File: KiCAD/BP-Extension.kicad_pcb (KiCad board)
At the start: 2 copper layers, 19.8 x 49.3 mm, 7 parts, among them P1 CONN_01X06, SW1 SW_Push, U1 BP, U2 RFM69

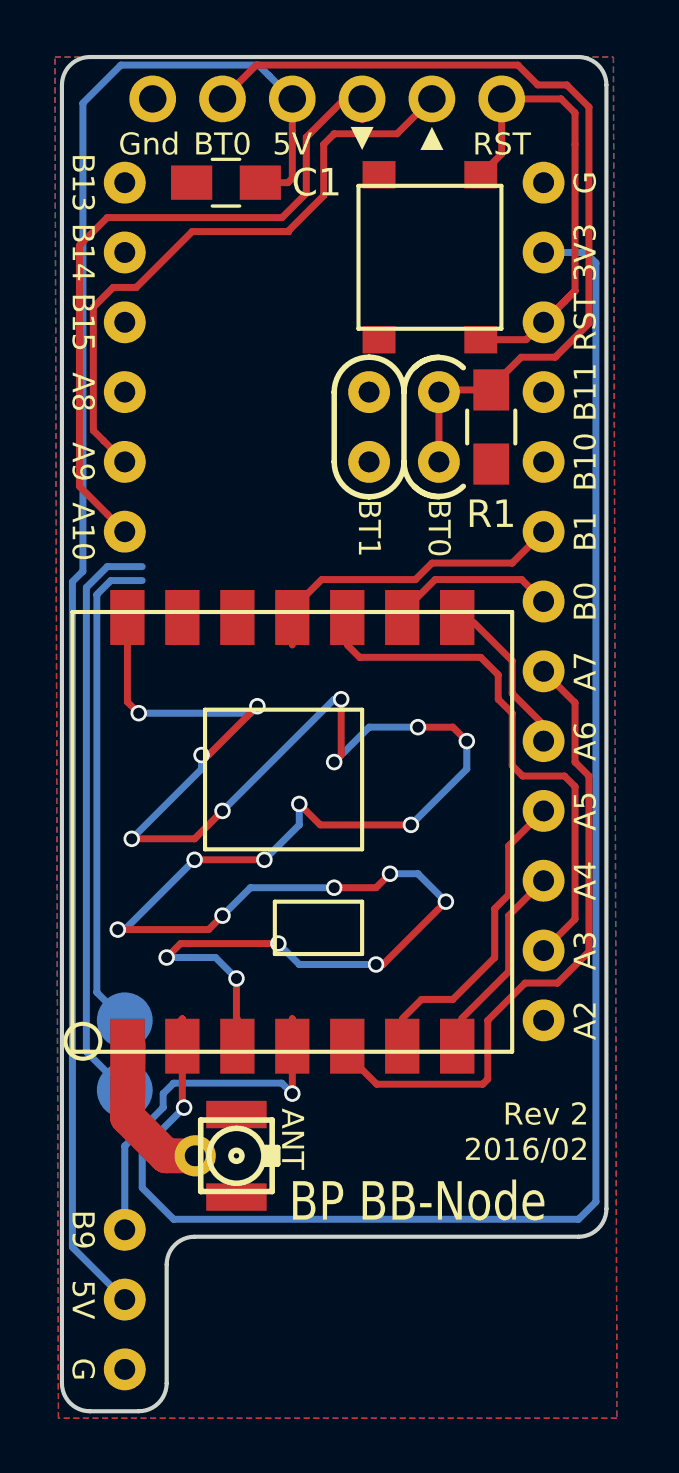
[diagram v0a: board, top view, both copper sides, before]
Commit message: On the way to rev2
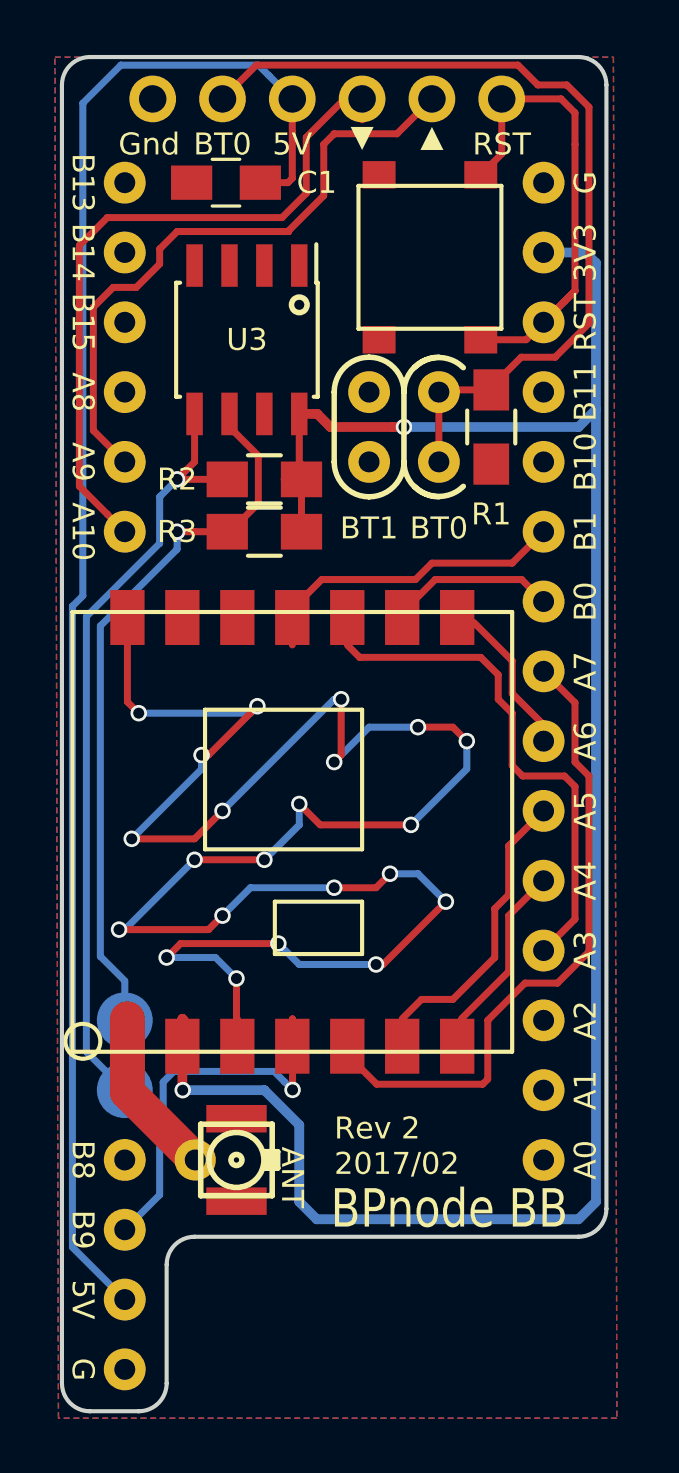
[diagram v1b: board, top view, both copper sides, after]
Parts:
- added R2: R, Resistors_SMD:R_0805_HandSoldering, F.Cu at (146.1, 94.6)
- added R3: R, Resistors_SMD:R_0805_HandSoldering, F.Cu at (146.1, 96.5)
- added U3: M24M02-DR, Housings_SOIC:SOIC-8_3.9x4.9mm_Pitch1.27mm, F.Cu at (145.4, 89.5)
- moved AE1 0.15 mm to (145.0, 119.4)
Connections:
- U1 pad PB6: (no net) -> SCL
- U1 pad PB7: (no net) -> SDA
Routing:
- net (no net): track 39.0 -> 0.00 mm
- net SDA: track 0.00 -> 28.6 mm, vias 0 -> 1
- net SCL: track 0.00 -> 26.5 mm, vias 0 -> 1
- net +3V3: track 60.4 -> 74.3 mm, vias 1 -> 2
- net DIO3: track 14.9 -> 13.7 mm
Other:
- net class Ant added: clearance 0.254, trace_width 1.27, via_dia 0.6, via_drill 0.4
- net class Power added: clearance 0.254, trace_width 0.3556, via_dia 0.6, via_drill 0.4
- board text added: "A0"
- board text added: "A1"
- board text added: "B8"
- board text added: "BPnode BB"
- board text added: "Rev 2 2017/02"
- board text removed: "BP BB-Node"
- board text removed: "Rev 2 2016/02"
